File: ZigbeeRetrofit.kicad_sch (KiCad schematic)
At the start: 24 parts, among them J1 110990030, J2 U.FL-R-SMT-1(10), J3 TC2050-IDC-NL, U1 CC2531F256RHAT, U2 SPX3819M5-L-3-3, Y1 32 Mhz, Y2 ECS-.327-12.5-34RR-TR

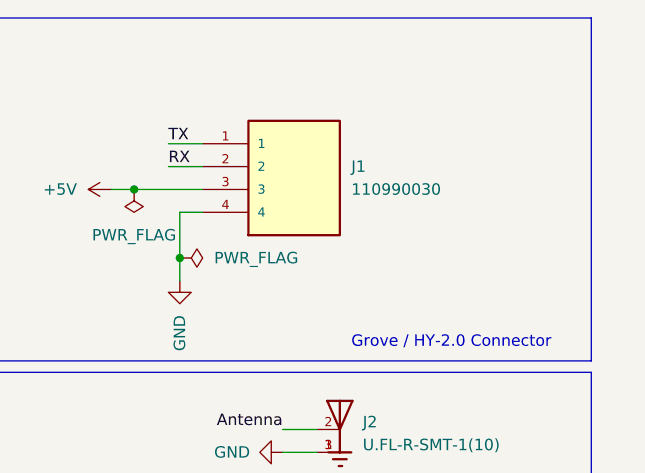
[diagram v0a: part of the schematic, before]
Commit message: Updated layout with 3d models
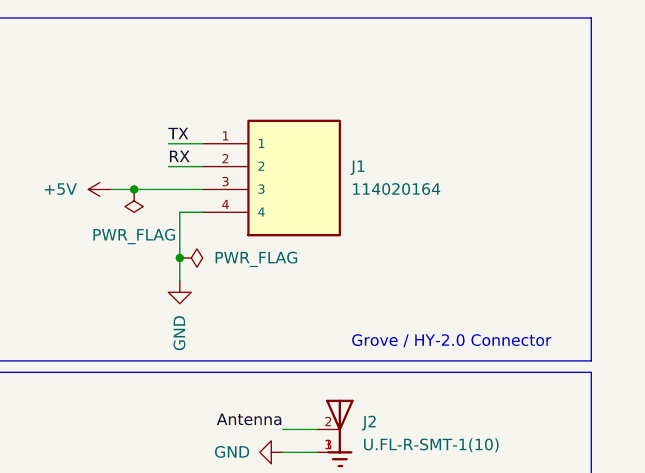
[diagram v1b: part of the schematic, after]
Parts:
- J1: value 110990030 -> 114020164
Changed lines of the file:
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@@
       (effects (font (size 1.27 1.27)) (justify left))
     )
-    (property "Value" "110990030" (id 1) (at 256.54 33.0199 0)
+    (property "Value" "114020164" (id 1) (at 256.54 33.0199 0)
       (effects (font (size 1.27 1.27)) (justify left))
     )
@@
     )
     (path "/8e4e635d-33a0-4932-856a-6a690a34c395"
-      (reference "J1") (unit 1) (value "110990030") (footprint "110990030:SEEED_110990030")
+      (reference "J1") (unit 1) (value "114020164") (footprint "110990030:SEEED_110990030")
     )
     (path "/33aac899-fc0a-4e6d-a4e5-d2f7cbb5983c"
